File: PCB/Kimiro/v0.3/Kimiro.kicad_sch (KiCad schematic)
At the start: 26 parts, among them J1 USB_C_Left, J2 Left, J3 Right, J4 , J5 , J6 , Q1 AO3407, U1 TP4054, U2 MS88FS3, U3 XC6220B331MR

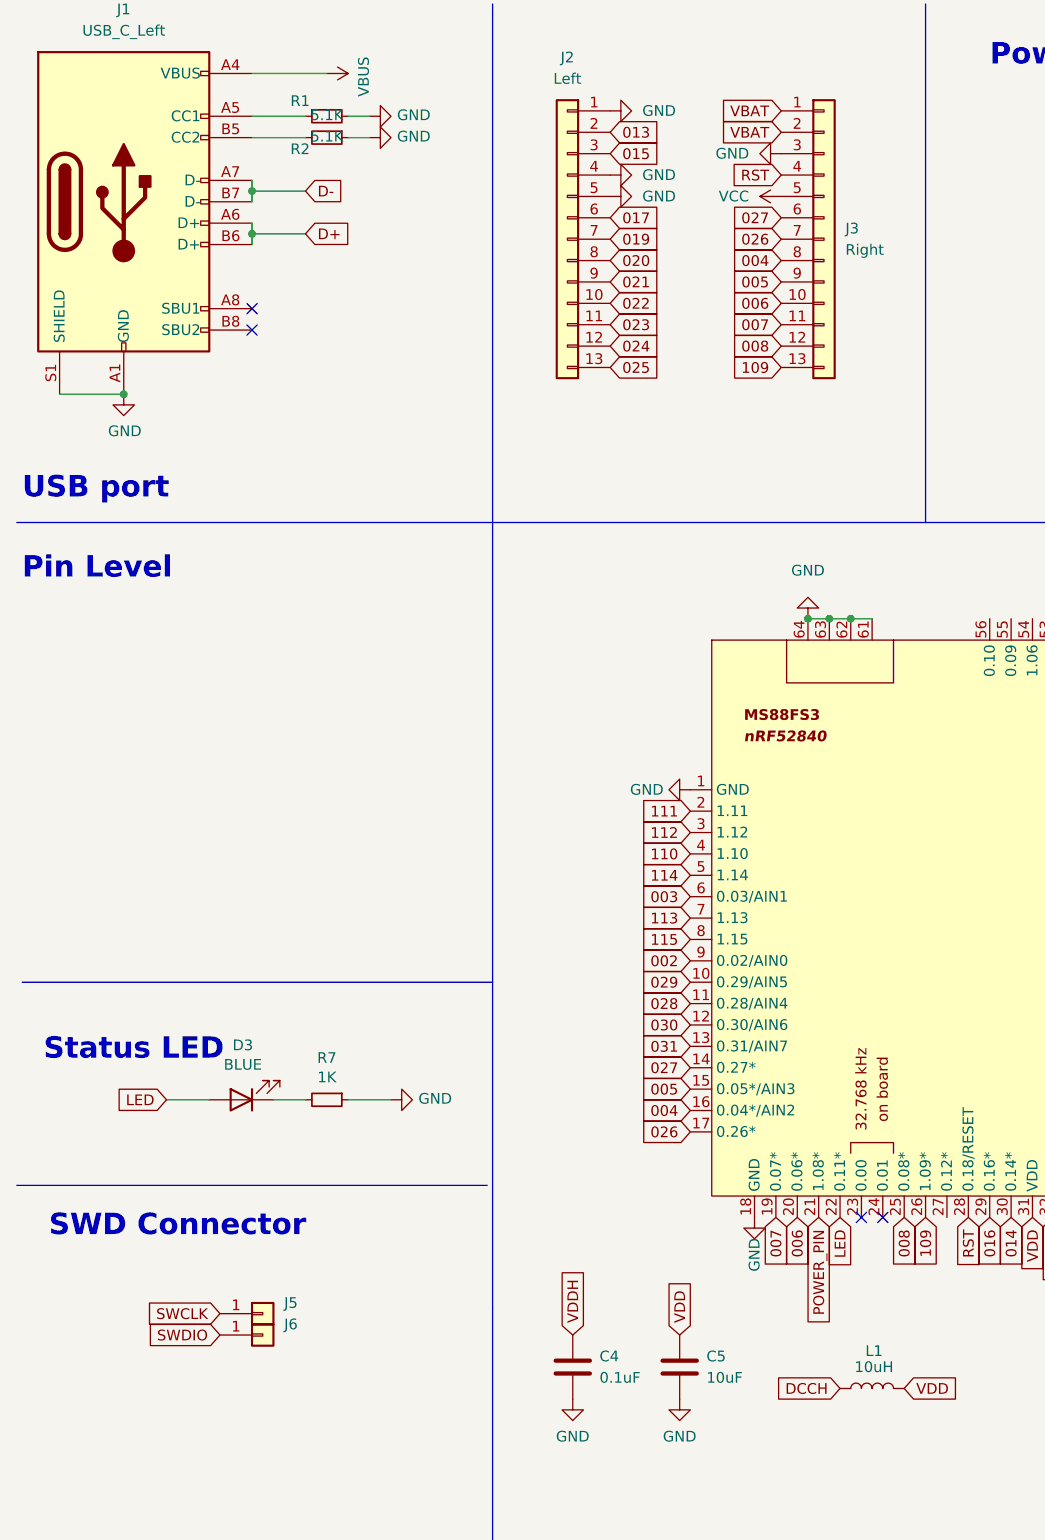
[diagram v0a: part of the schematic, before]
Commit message: Update bootloader.hex, flashbed.kicad_pcb, and 54 more files...
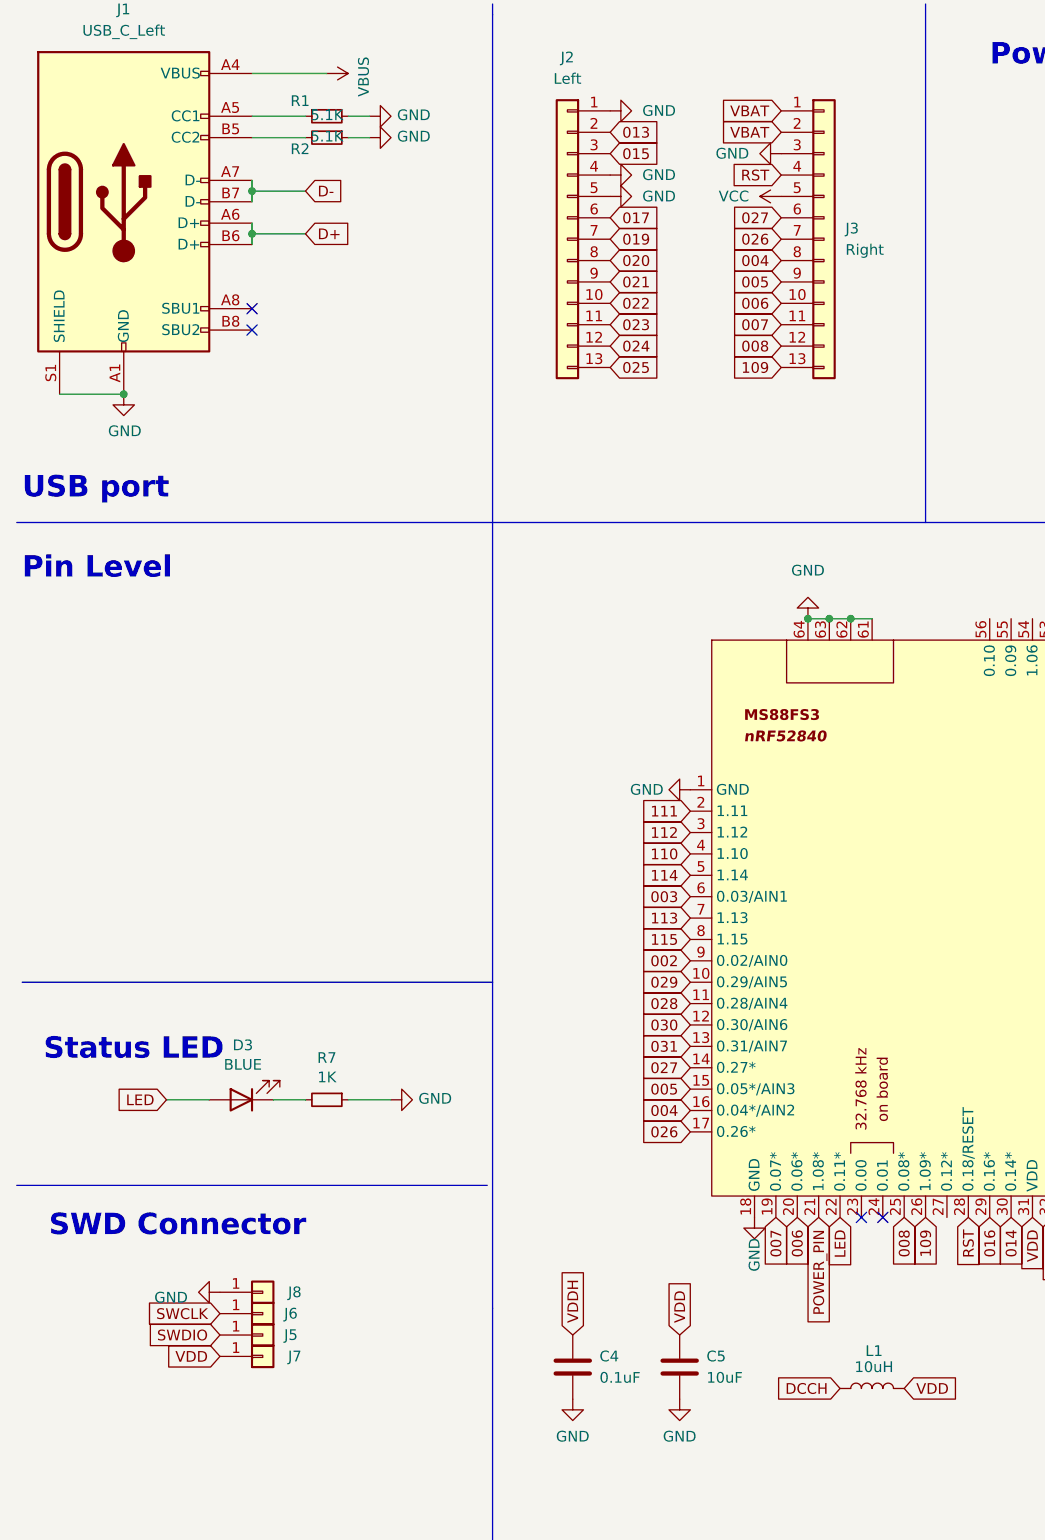
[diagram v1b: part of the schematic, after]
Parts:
- added J7, J8: (no value), Kimiro-library:Conn_1x01, symbol Connector_Generic:Conn_01x01
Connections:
- net GND: now also J8.1 (Pin_1)
- net SWCLK: now also J6.1 (Pin_1); no longer J5.1 (Pin_1)
- net SWDIO: now also J5.1 (Pin_1); no longer J6.1 (Pin_1)
- net VDD: now also J7.1 (Pin_1)
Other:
- moved on the sheet: J5, J6
